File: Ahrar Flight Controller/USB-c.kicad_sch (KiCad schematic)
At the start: 9 parts, among them J9 USB4105-GF-A-120, U4 TPD2EUSB30DRTR

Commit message: .
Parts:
- R13, R5, R6: footprint Capacitor_SMD:C_0402_1005Metric -> Resistor_SMD:R_0402_1005Metric

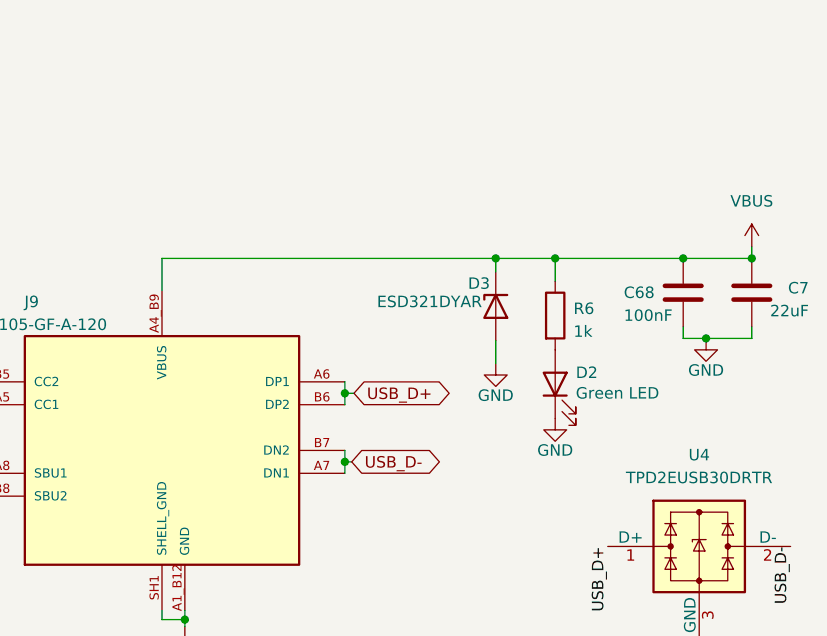
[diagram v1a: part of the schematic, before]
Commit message: .
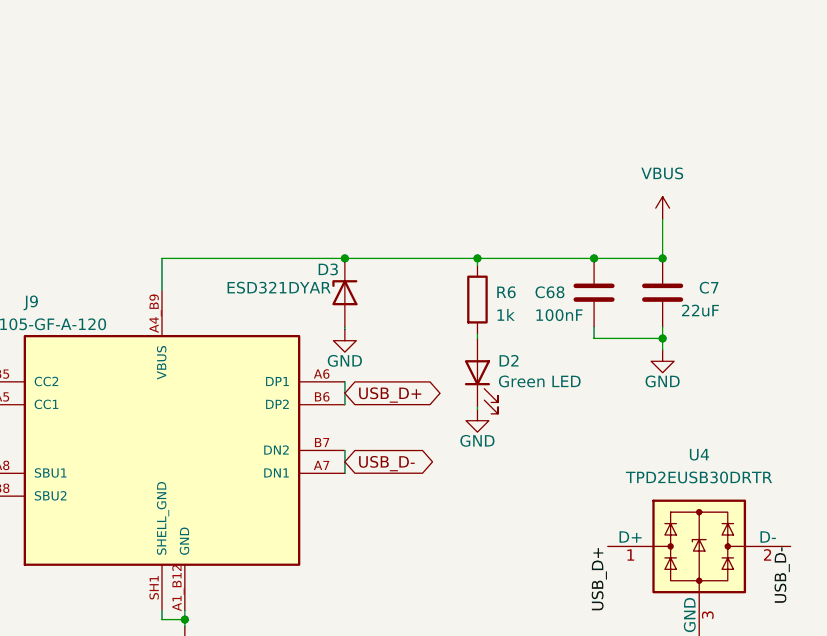
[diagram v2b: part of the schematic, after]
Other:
- moved on the sheet: C68, C7, D2, D3, R6
